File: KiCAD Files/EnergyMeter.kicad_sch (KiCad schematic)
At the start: 40 parts, among them J1 Screw_Terminal_AC, J2 Conn_01x05, SW1 SW_Push, U1 AMS1117-3.3, U2 ESP-12F, U3 HLW8032

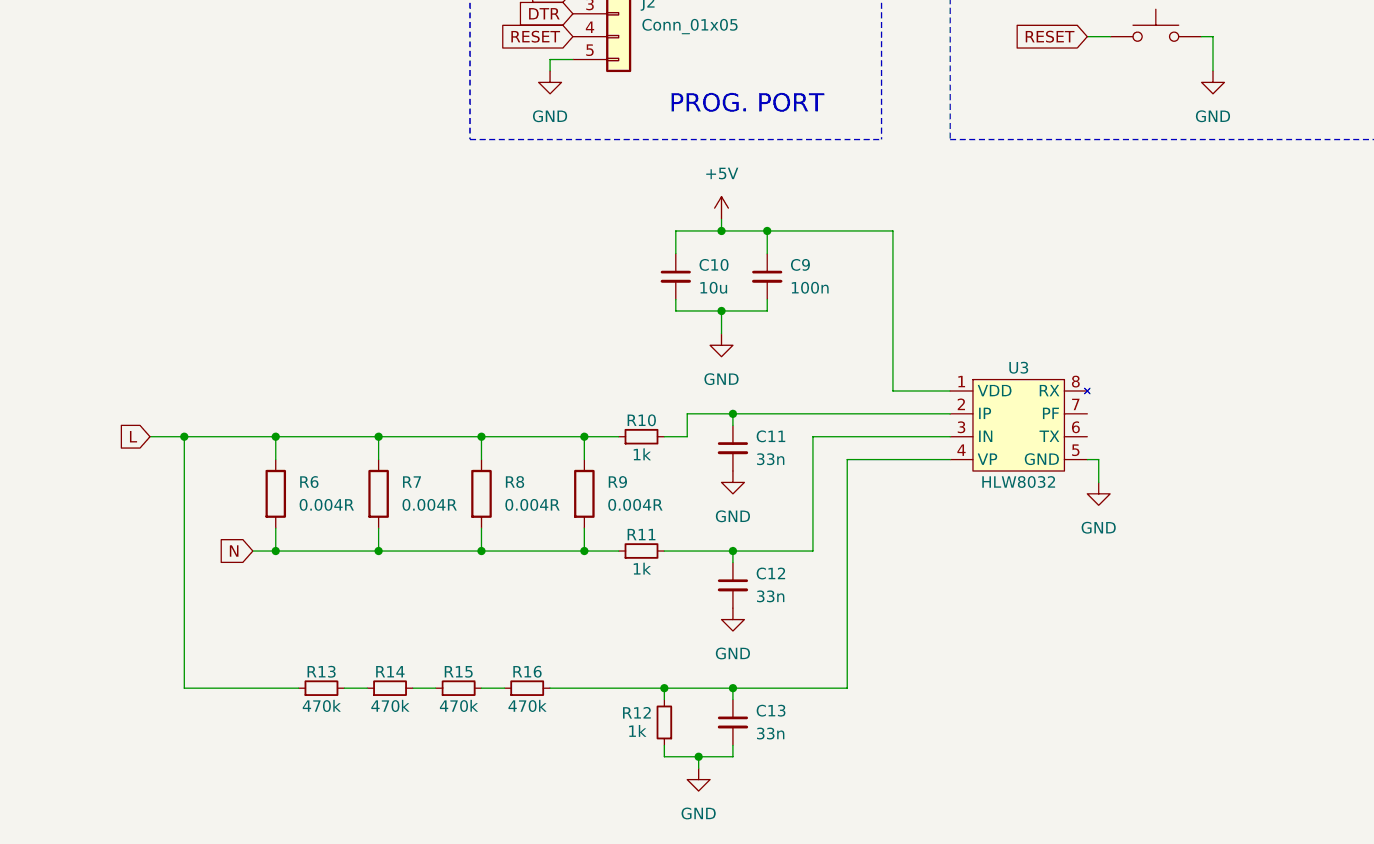
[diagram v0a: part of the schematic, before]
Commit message: Schematic update
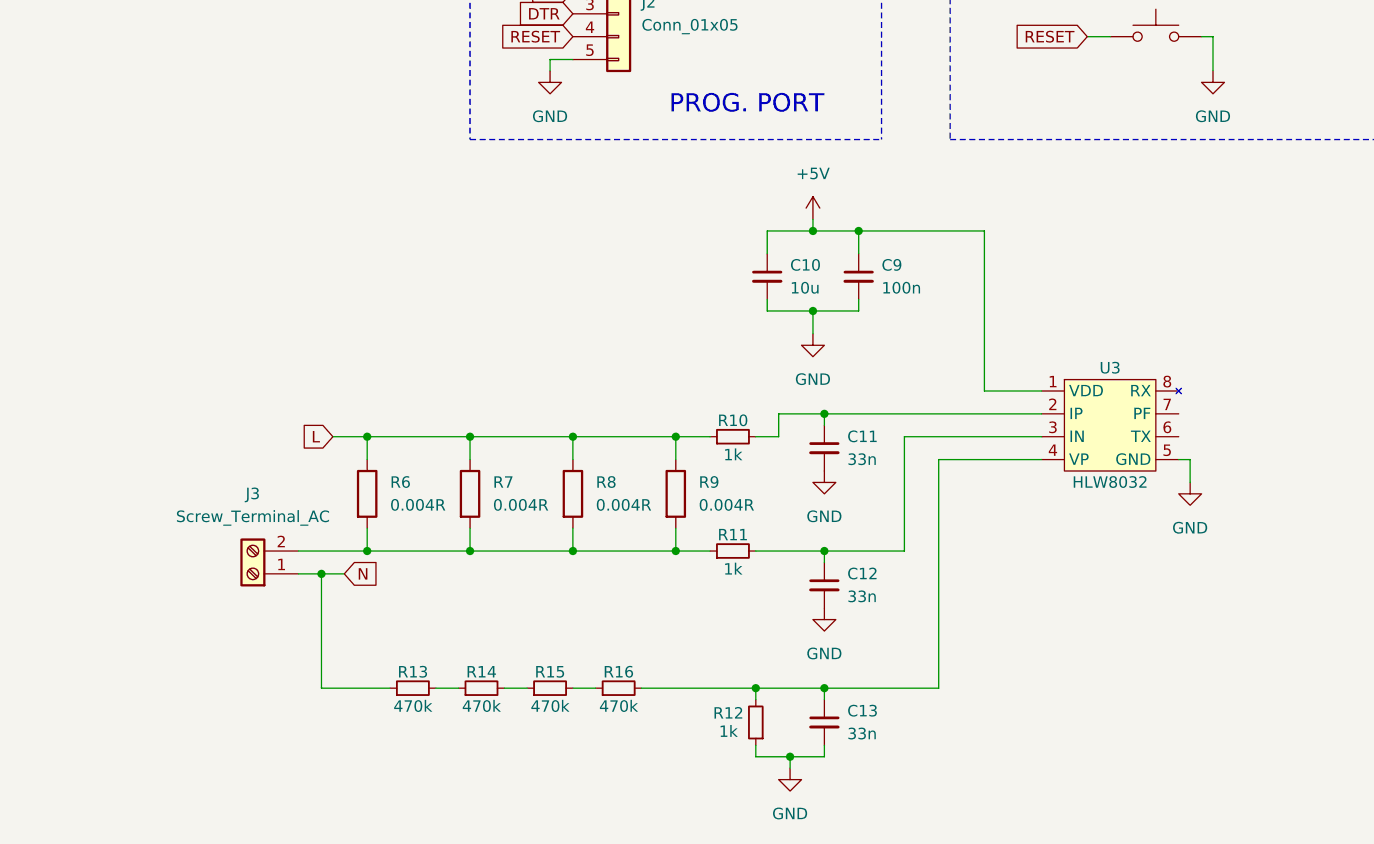
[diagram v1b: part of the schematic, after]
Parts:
- added J3: Screw_Terminal_AC, symbol Connector:Screw_Terminal_01x02
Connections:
- net L: no longer R13.1
- net N: now also R13.1, J3.1 (Pin_1); no longer R11.1, R6.2, R7.2, R8.2, R9.2
- new net: J3.2 (Pin_2), R11.1, R6.2, R7.2, R8.2, R9.2
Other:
- moved on the sheet: C10, C11, C12, C13, C9, R10, R11, R12, R13, R14, R15, R16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

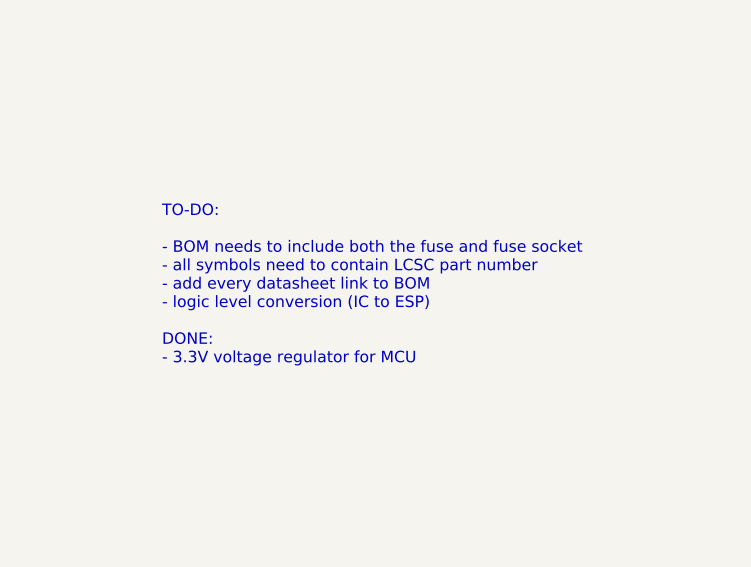
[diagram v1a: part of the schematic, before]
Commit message: TO-DO update
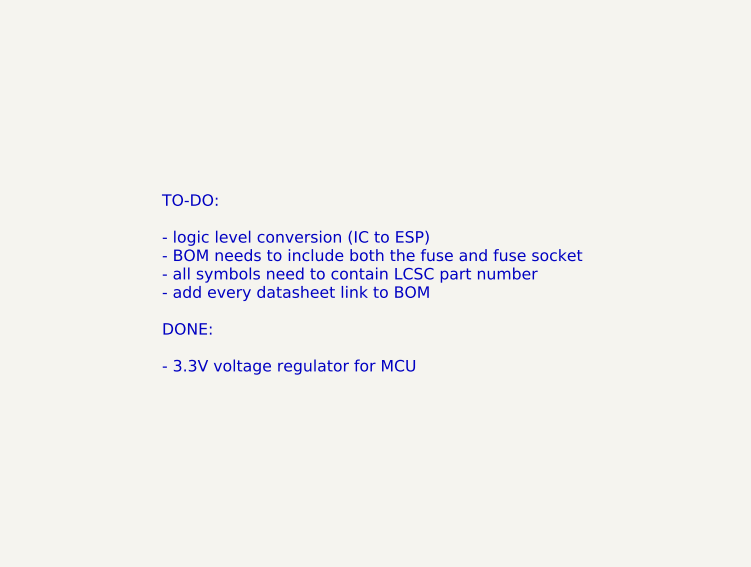
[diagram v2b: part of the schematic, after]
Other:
- note added: "TO-DO: - logic level conversion (IC to ESP) - BOM needs to include both the fuse and fuse socket - all symbols need to contain LCSC part number - add every datasheet link to BOM DONE: - 3.3V voltage regulator for MCU"
- note removed: "TO-DO: - BOM needs to include both the fuse and fuse socket - all symbols need to contain LCSC part number - add every datasheet link to BOM - logic level conversion (IC to ESP) DONE: - 3.3V voltage regulator for MCU"
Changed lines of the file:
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@@
 		)
 	)
-	(text "TO-DO:\n\n- BOM needs to include both the fuse and fuse socket\n- all symbols need to contain LCSC part number\n- add every datasheet link to BOM\n- logic level conversion (IC to ESP)\n\nDONE:\n- 3.3V voltage regulator for MCU\n"
+	(text "TO-DO:\n\n- logic level conversion (IC to ESP)\n- BOM needs to include both the fuse and fuse socket\n- all symbols need to contain LCSC part number\n- add every datasheet link to BOM\n\nDONE:\n\n- 3.3V voltage regulator for MCU\n"
 		(exclude_from_sim no)
 		(at 226.822 155.194 0)

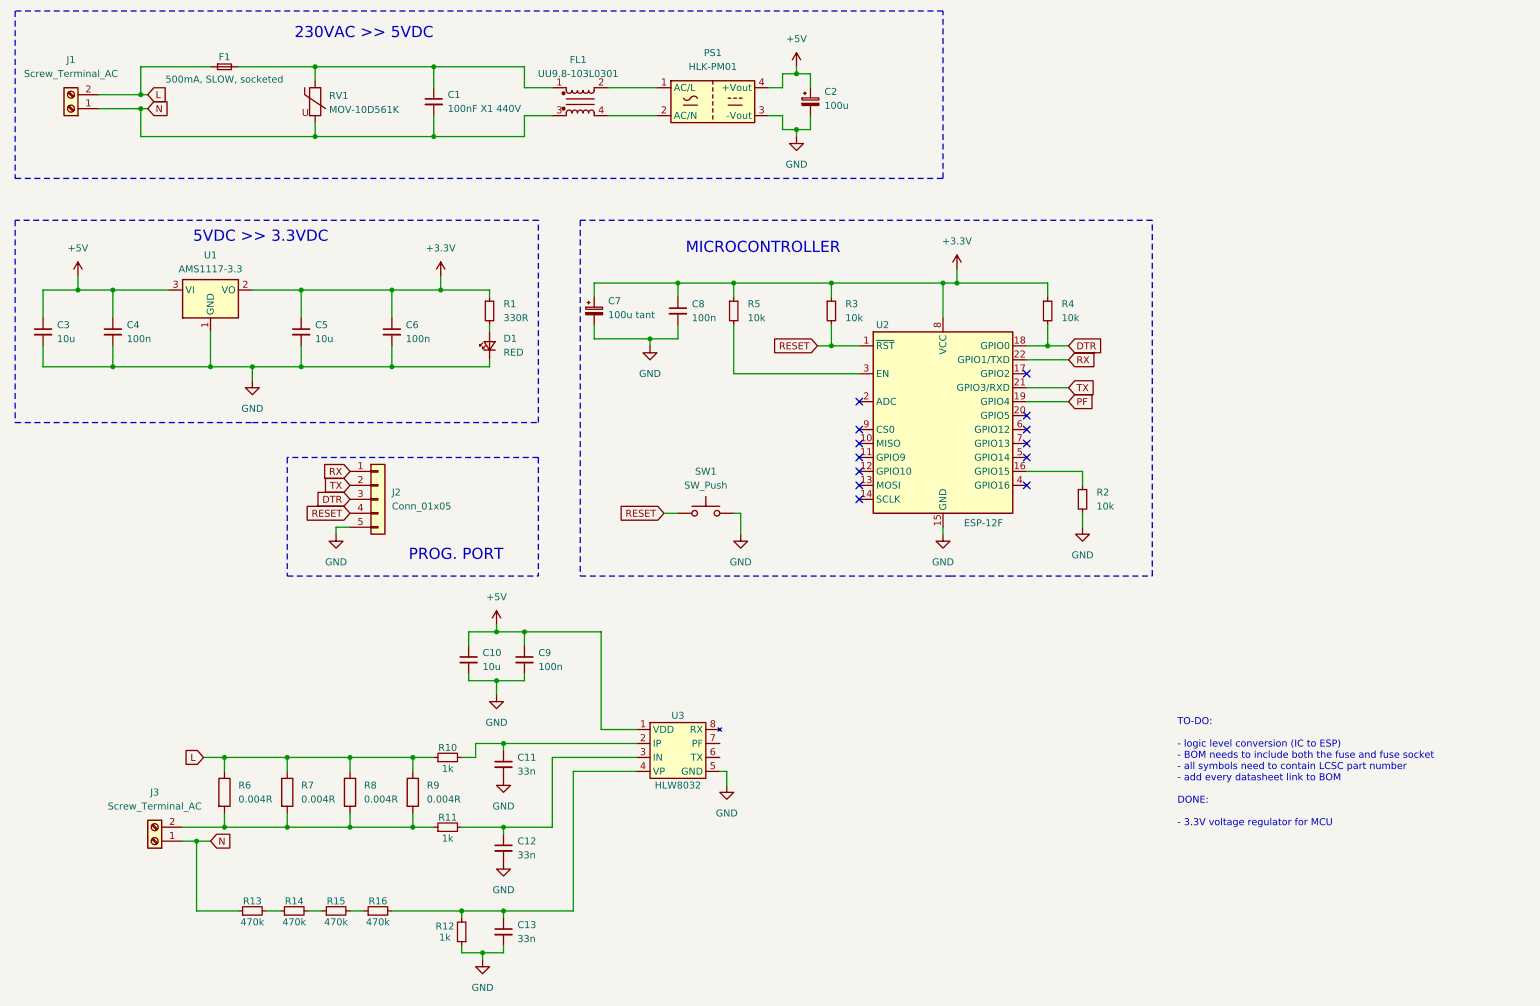
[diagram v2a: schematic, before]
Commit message: Schematic update
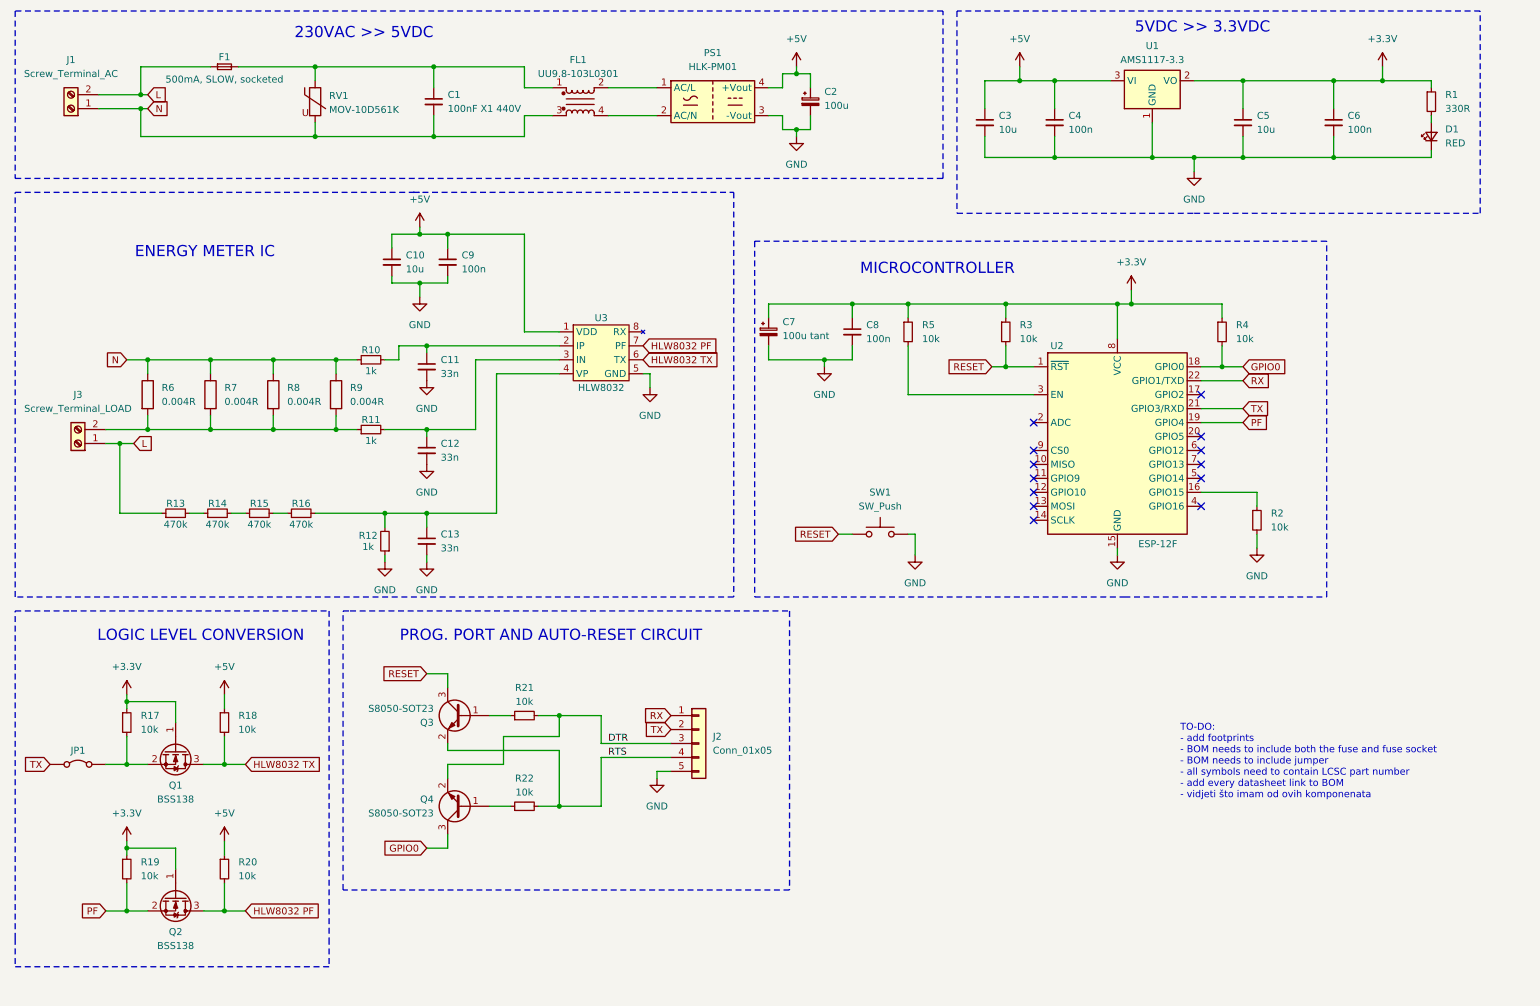
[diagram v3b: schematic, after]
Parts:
- added JP1: Jumper_2_Bridged, symbol Jumper:Jumper_2_Bridged
- added Q1, Q2: BSS138, Package_TO_SOT_SMD:SOT-23, symbol Transistor_FET:BSS138
- added Q3, Q4: S8050-SOT23, Package_TO_SOT_SMD:SOT-23, symbol Symbol_Library:S8050-SOT23
- added R17, R18, R19, R20, R21, R22: 10k, Resistor_SMD:R_0805_2012Metric, symbol Device:R_Small
- C1: footprint (none) -> Capacitor_THT:C_Rect_L18.0mm_W8.0mm_P15.00mm_FKS3_FKP3; LCSC Part # C105712 -> C93321
- C10, C3, C5: footprint (none) -> Capacitor_SMD:C_1206_3216Metric
- C11, C12, C13, C4, C6, C8, C9: footprint (none) -> Capacitor_SMD:C_0805_2012Metric
- C2: footprint (none) -> Capacitor_THT:CP_Radial_D8.0mm_P3.50mm
- C7: footprint (none) -> Capacitor_Tantalum_SMD:CP_EIA-7343-15_Kemet-W
- D1: footprint (none) -> LED_SMD:LED_0805_2012Metric
- J3: value Screw_Terminal_AC -> Screw_Terminal_LOAD
- R1, R10, R11, R12, R13, R14, R15, R16, R2, R3, R4, R5: footprint (none) -> Resistor_SMD:R_0805_2012Metric
- U3: footprint (none) -> Package_SO:SOP-8_3.9x4.9mm_P1.27mm; LCSC Part # (none) -> C128023; LCSC Part# C128023 -> (none)
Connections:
- net +3.3V: now also Q1.1 (G), Q2.1 (G), R17.1, R19.1
- net +5V: now also R18.1, R20.1
- net DTR: now also Q4.2 (E), R21.2; no longer R4.2, U2.18 (GPIO0)
- net L: now also J3.1 (Pin_1), R13.1; no longer R10.1, R6.1, R7.1, R8.1, R9.1
- net N: now also R10.1, R6.1, R7.1, R8.1, R9.1; no longer J3.1 (Pin_1), R13.1
- net PF: now also Q2.2 (S), R19.2
- net RESET: now also Q3.3 (C); no longer J2.4 (Pin_4)
- net TX: now also JP1.1 (A)
- net HLW8032 TX: now reaches U3.6 (TX)
- net HLW8032 TX: now also Q1.3 (D), R18.2
- net HLW8032 PF: now reaches U3.7 (PF)
- net HLW8032 PF: now also Q2.3 (D), R20.2
- new net: JP1.2 (B), Q1.2 (S), R17.2
- new net: Q3.1 (B), R21.1
- new net: Q4.1 (B), R22.1
- new net GPIO0: Q4.3 (C), R4.2, U2.18 (GPIO0)
- new net RTS: J2.4 (Pin_4), Q3.2 (E), R22.2
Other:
- note added: "ENERGY METER IC"
- note added: "LOGIC LEVEL CONVERSION"
- note added: "PROG. PORT AND AUTO-RESET CIRCUIT"
- note added: "TO-DO: - add footprints - BOM needs to include both the fuse and fuse socket - BOM needs to include jumper - all symbols need to contain LCSC part number - add every datasheet link to BOM - vidjeti što imam od ovih komponenata"
- note removed: "PROG. PORT"
- note removed: "TO-DO: - logic level conversion (IC to ESP) - BOM needs to include both the fuse and fuse socket - all symbols need to contain LCSC part number - add every datasheet link to BOM DONE: - 3.3V voltage regulator for MCU"
- moved on the sheet: C10, C11, C12, C13, C3, C4, C5, C6, C7, C8, C9, D1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
